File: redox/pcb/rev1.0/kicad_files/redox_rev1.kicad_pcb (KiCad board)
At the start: 2 copper layers, 162.2 x 126.5 mm, 86 parts, among them K0 KEYSW, K1 KEYSW, K10 KEYSW, K11 KEYSW, K12 KEYSW, K13 KEYSW, K14 KEYSW, K15 KEYSW, K16 KEYSW, K2 KEYSW, K20 KEYSW, K21 KEYSW, K22 KEYSW, K23 KEYSW, K24 KEYSW, K25 KEYSW, K26 KEYSW, K3 KEYSW, K30 KEYSW, K31 KEYSW, K32 KEYSW, K33 KEYSW, K34 KEYSW, K35 KEYSW, K36 KEYSW, K4 KEYSW, K40 KEYSW, K41 KEYSW, K42 KEYSW, K43 KEYSW, K44 KEYSW, K45 KEYSW, K46 KEYSW, K5 KEYSW, K6 KEYSW, U1 ProMicro

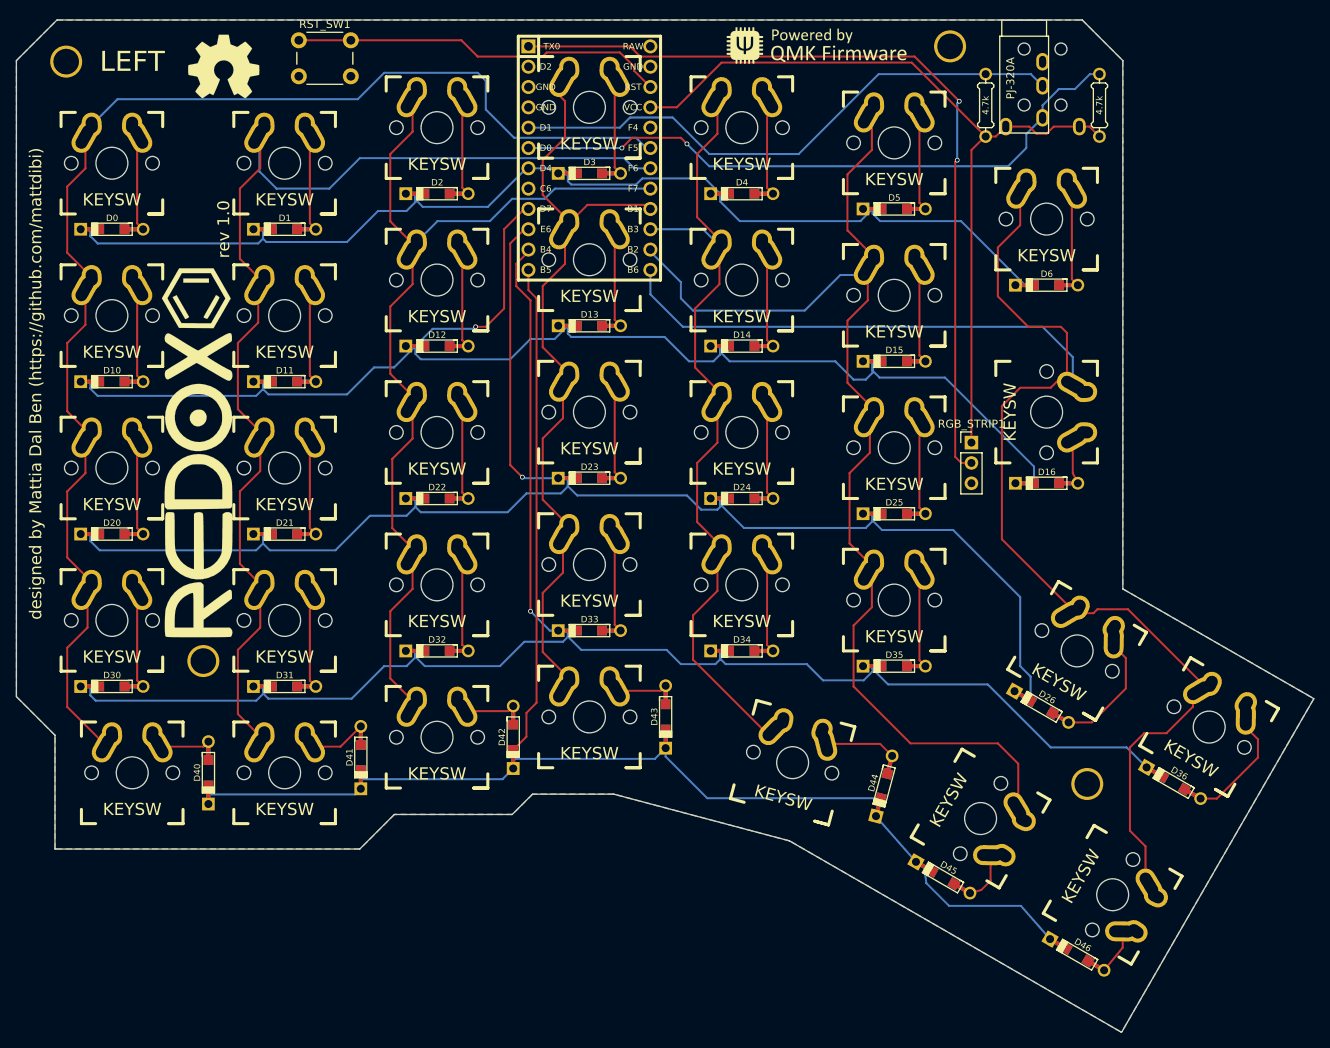
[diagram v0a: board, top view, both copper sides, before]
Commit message: re-redox changes pcb changes
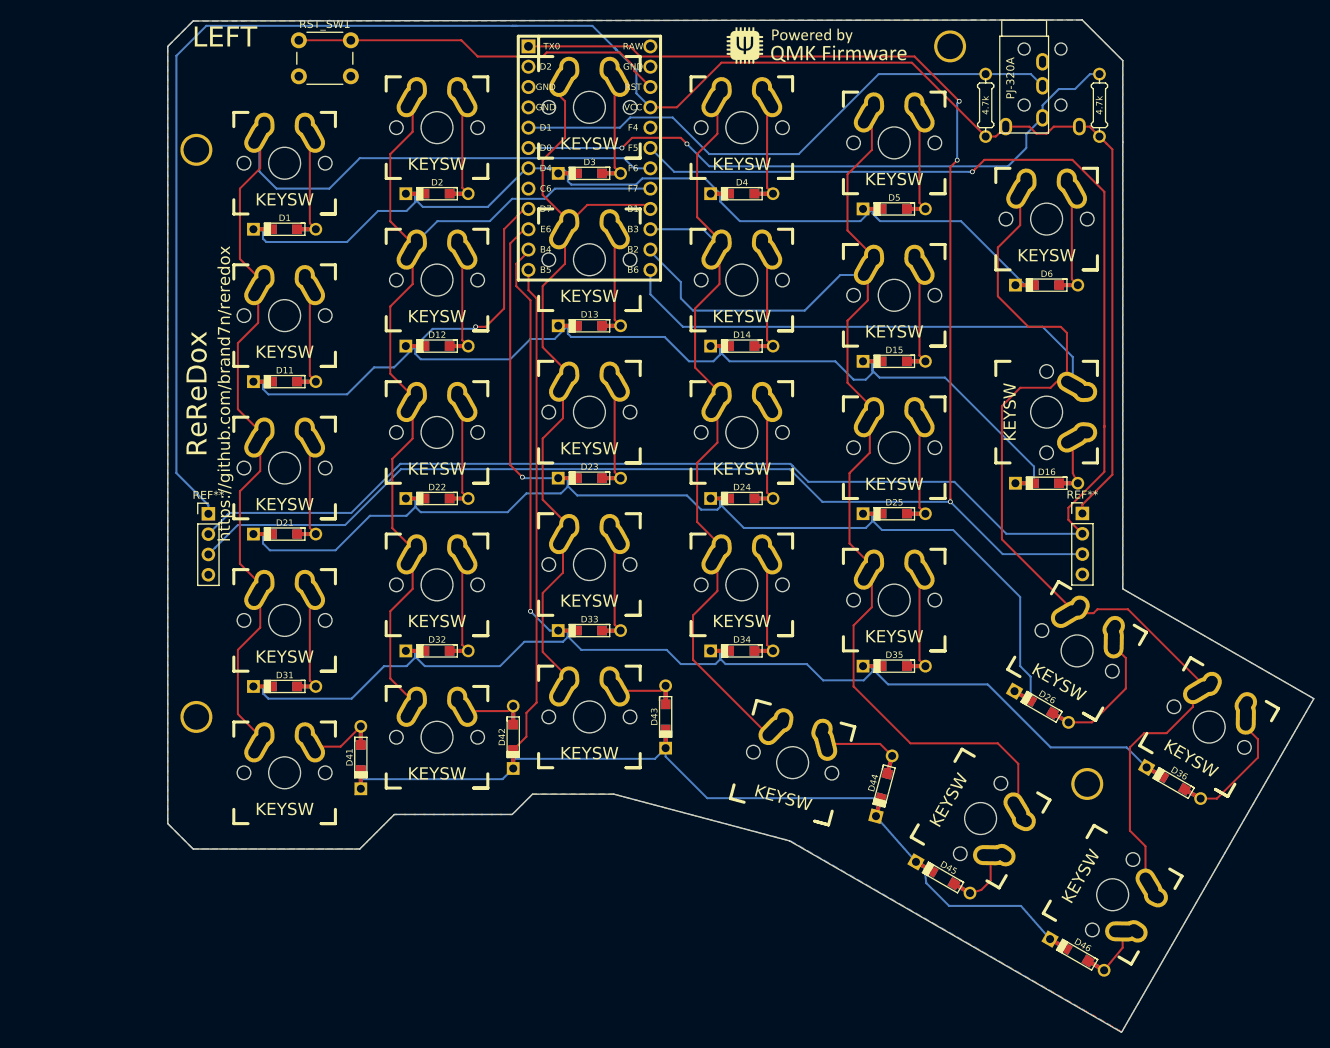
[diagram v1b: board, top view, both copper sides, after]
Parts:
- removed D0, D10, D20, D30, D40: D, Keebio-Parts:Diode-dual
- removed the G*** at (102.2, 102.9)
- removed the G*** at (102.2, 102.2)
- removed K0, K10, K20, K30: KEYSW, myparts:Mx_Alps_125-dualside
- removed K40: KEYSW, canadian_footprints:Mx_Alps_100-dualside
- removed REF*** (x2): OSHW-Logo2_14.6x12mm_SilkScreen, Symbols:OSHW-Symbol_8.9x8mm_SilkScreen
- removed RGB_STRIP1: Conn_01x03, Pin_Headers:Pin_Header_Straight_1x03_Pitch2.54mm
- added REF**: PinHeader_1x04_P2.54mm_Vertical, Connector_PinHeader_2.54mm:PinHeader_1x04_P2.54mm_Vertical, F.Cu at (212.8, 110.5)
- added REF**: PinHeader_1x04_P2.54mm_Vertical, Connector_PinHeader_2.54mm:PinHeader_1x04_P2.54mm_Vertical, F.Cu at (103.5, 110.5)
- moved HOLE_M3 19.7 mm to (102.0, 65.0)
- moved HOLE_M3 7.04 mm to (102.0, 135.9)
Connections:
- HOLE_M3 pad 1: (no net) -> GND (x4)
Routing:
- net VCC: track 103.1 -> 240.0 mm
- net rgb_data: track 103.7 -> 225.3 mm, vias 2 -> 3
- net col0: track 167.6 -> 223.2 mm, vias 0 -> 1
- net row3: track 207.9 -> 184.5 mm
- net row2: track 188.9 -> 165.6 mm
- net row1: track 169.3 -> 146.1 mm
- net row0: track 135.3 -> 112.3 mm
- net row4: track 189.3 -> 170.9 mm
- net Net-(D30-Pad2): track 11.8 -> 0.00 mm
- net Net-(D20-Pad2): track 11.8 -> 0.00 mm
- net Net-(D10-Pad2): track 11.8 -> 0.00 mm
- net Net-(D0-Pad2): track 11.8 -> 0.00 mm
- net Net-(D40-Pad2): track 6.63 -> 0.00 mm
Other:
- board size 162.2 x 126.5 mm -> 143.3 x 126.5 mm
- board text added: "ReReDox"
- board text added: "https://github.com/brand7n/reredox"
- board text removed: "designed by Mattia Dal Ben (https://github.com/mattdibi)"
- board text removed: "rev 1.0"
